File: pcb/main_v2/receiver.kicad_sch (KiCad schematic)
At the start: 13 parts, among them IC401 HMC374, IC402 RMS-30+

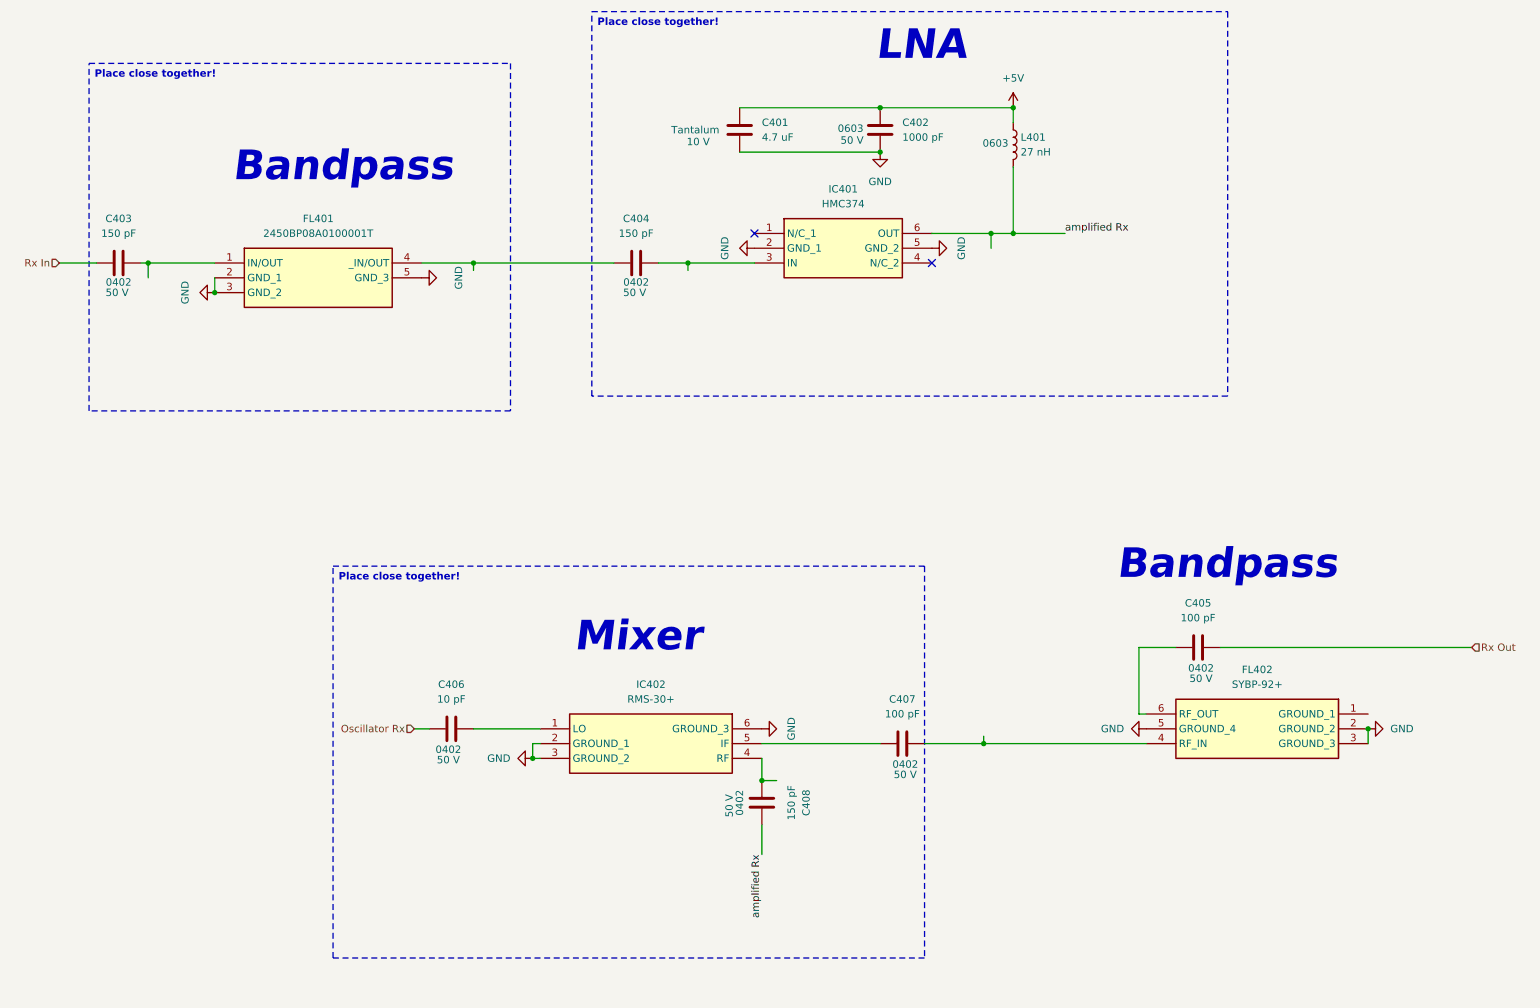
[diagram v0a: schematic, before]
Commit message: update bom
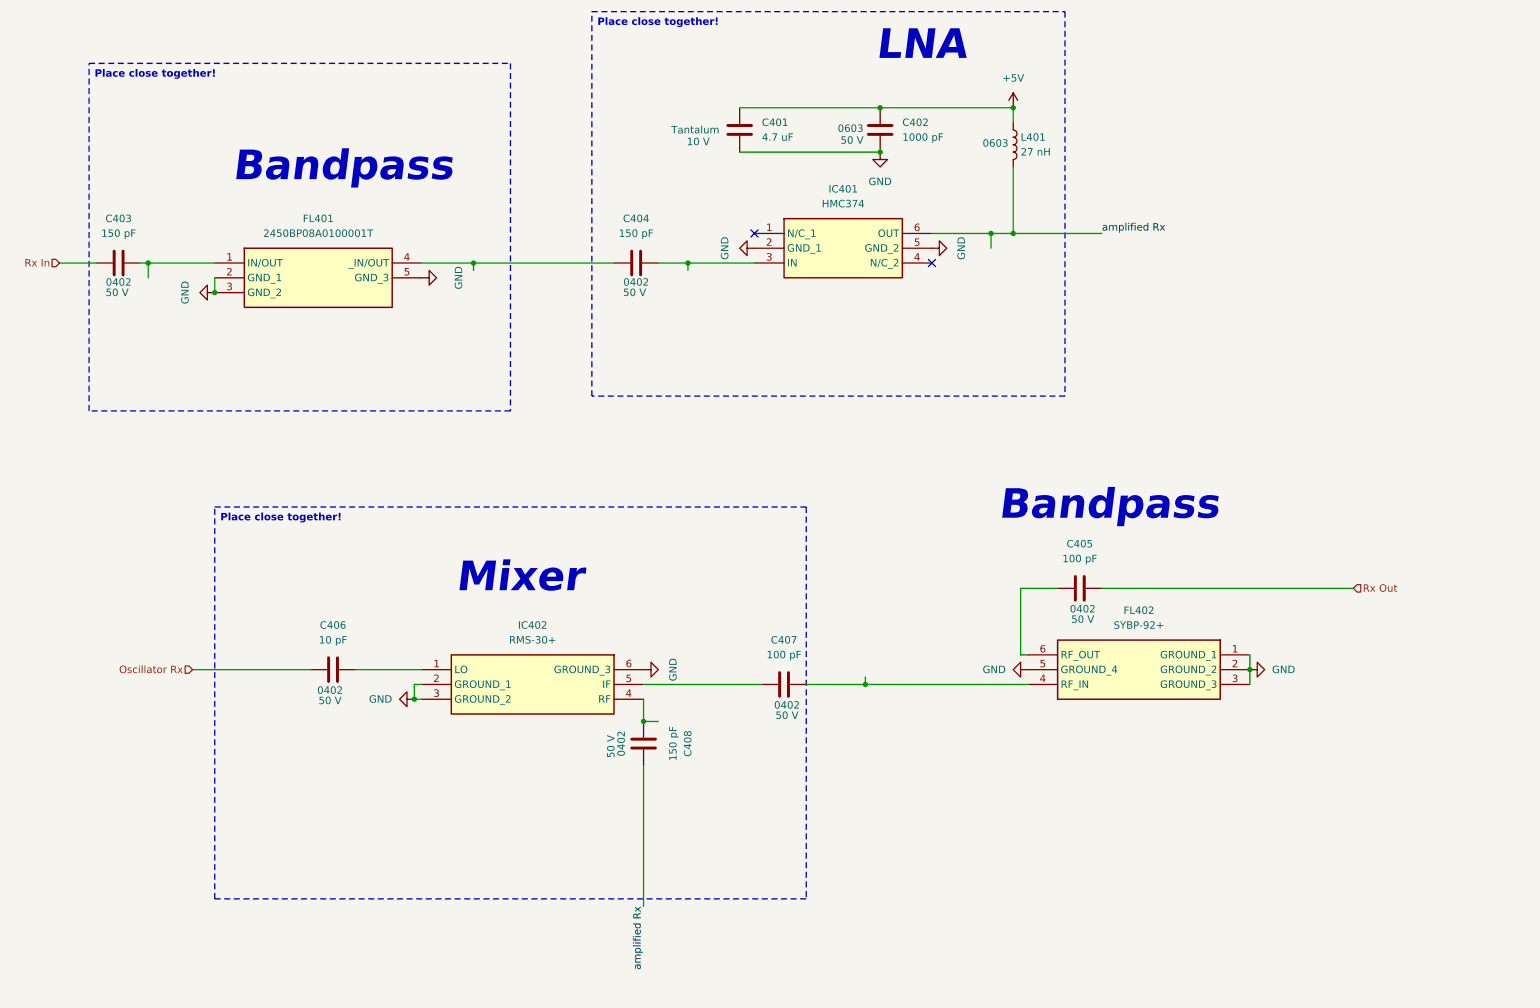
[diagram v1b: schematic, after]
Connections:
- net GND: now also FL402.1 (GROUND_1)
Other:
- moved on the sheet: C405, C406, C407, C408, FL402, IC402
